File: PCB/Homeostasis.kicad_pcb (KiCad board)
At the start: 2 copper layers, 109.5 x 98.8 mm, 46 parts, among them J1 USB_Connector, J2 ISP_Connector, J3 Fan_1, J4 Fan_2, J5 TPROBE_1, J6 TPROBE_2, J7 TPROBE_3, J8 TPROBE_4, J9 OLED, Q1 2N7002, Q2 2N7002, SW1 SW_Push, SW2 SW_Push, SW3 SW_Push, SW4 SW_Push, U2 ATmega328P-P, Y1 16MHz

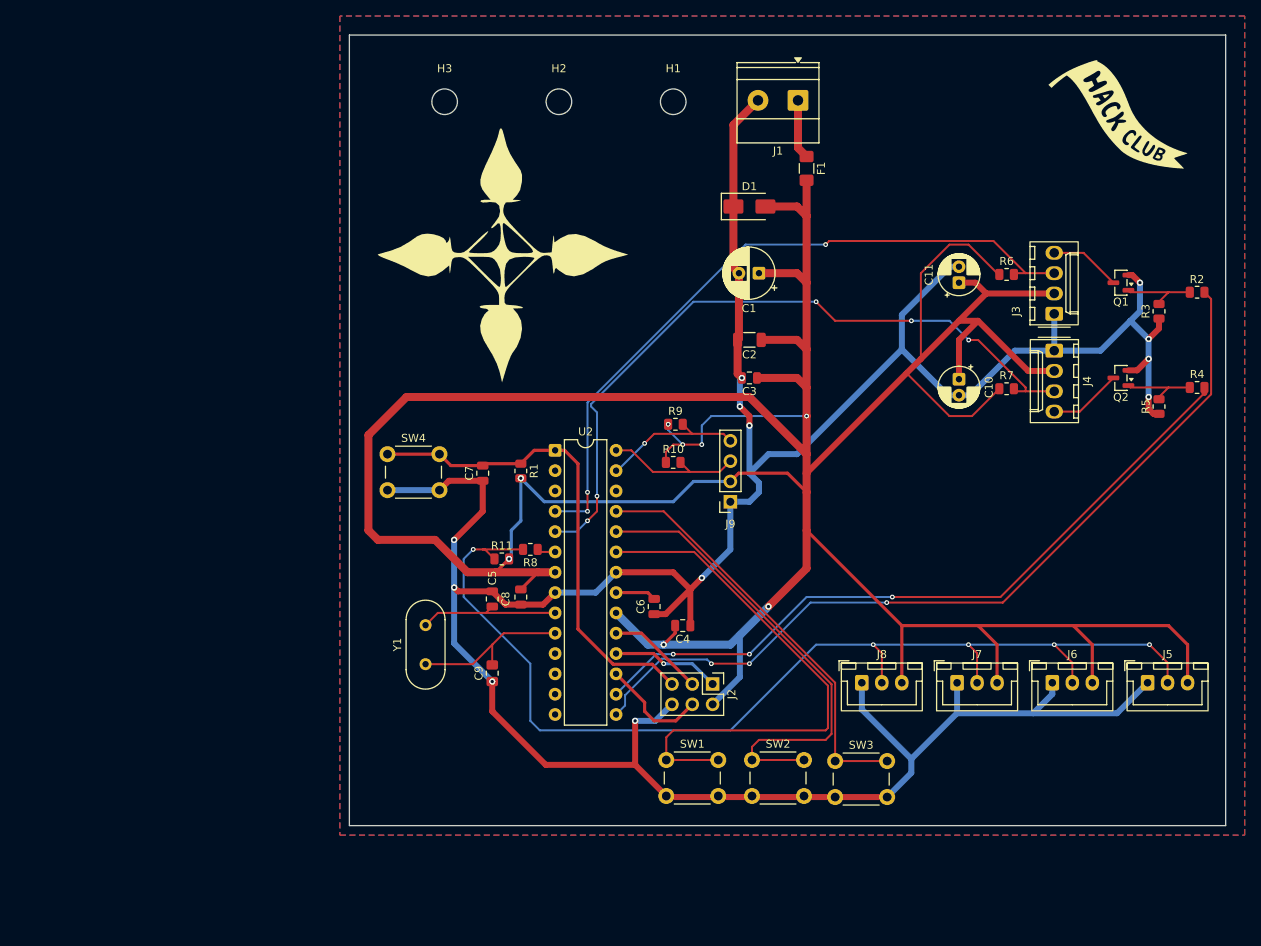
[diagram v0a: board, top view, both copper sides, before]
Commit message: PCB Final
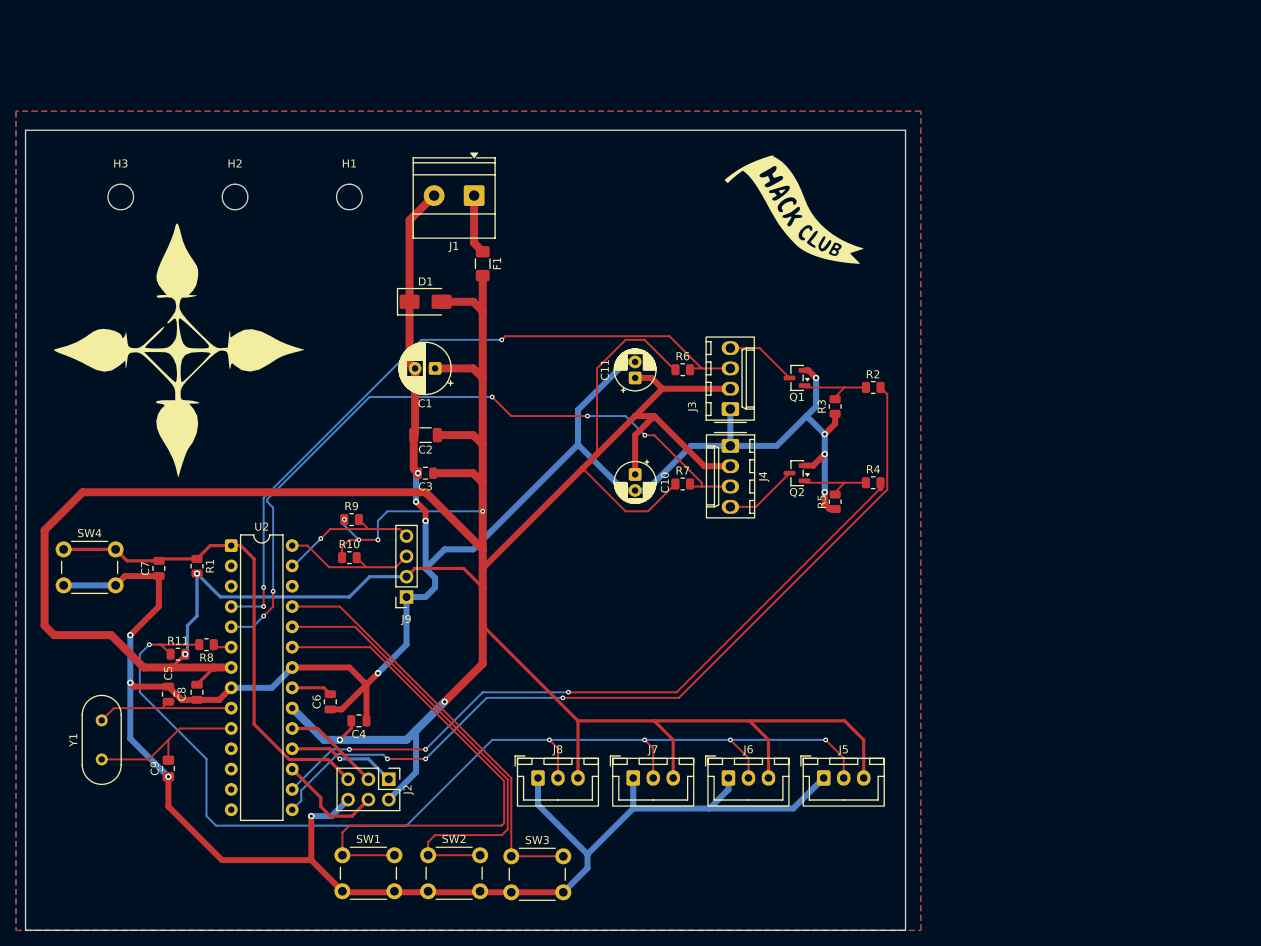
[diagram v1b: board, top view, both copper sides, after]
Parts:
- moved Q1 42.2 mm to (115.5, 54.8)
- moved Q2 42.2 mm to (115.5, 66.7)
- moved C1 42.2 mm to (70.2, 53.6)
- moved C4 42.2 mm to (60.7, 97.6)
- moved C5 42.2 mm to (40.5, 94.1)
- moved C7 42.2 mm to (35.7, 78.6)
- moved C8 42.2 mm to (36.9, 94.3)
- moved C9 42.2 mm to (36.9, 103.6)
- moved F1 42.2 mm to (76.2, 40.5)
- moved H1 42.2 mm to (59.5, 32.1)
- moved H3 42.2 mm to (31.0, 32.1)
- moved J1 42.2 mm to (75.1, 32.0)
- moved J2 42.2 mm to (64.5, 104.9)
- moved J5 42.2 mm to (118.8, 104.8)
- moved J6 42.2 mm to (106.9, 104.8)
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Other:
- board size 109.5 x 98.8 mm -> 110 x 100 mm
